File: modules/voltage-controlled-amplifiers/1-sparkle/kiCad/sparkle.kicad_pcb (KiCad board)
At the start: 2 copper layers, 90 x 111 mm, 83 parts, among them J1 OUT_1, J2 IN_1, J3 CV_1, J4 OUT_2, J5 IN_2, J6 CV_2, Q1 BC548, Q2 BC548, Q3 BC548, Q4 BC548, U1 TL074

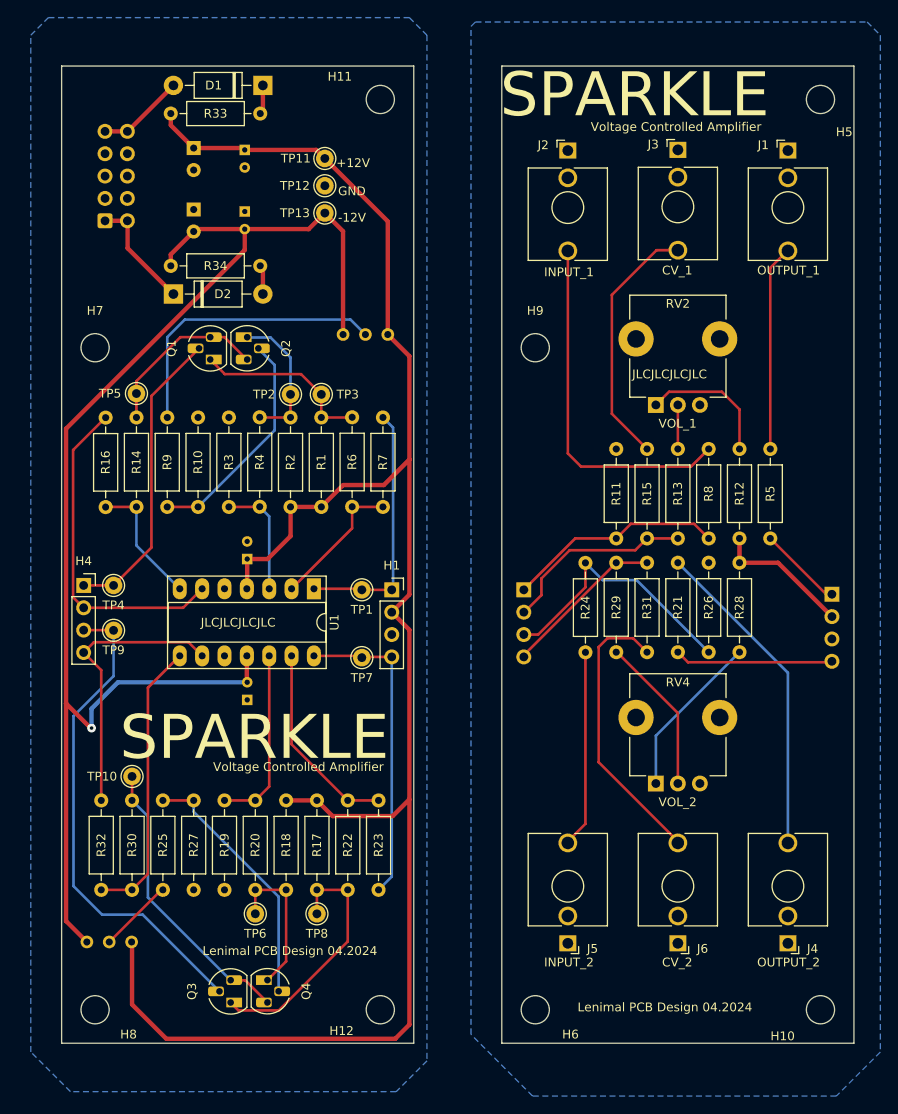
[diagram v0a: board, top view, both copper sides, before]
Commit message: add gerber files and ZIPs for V2
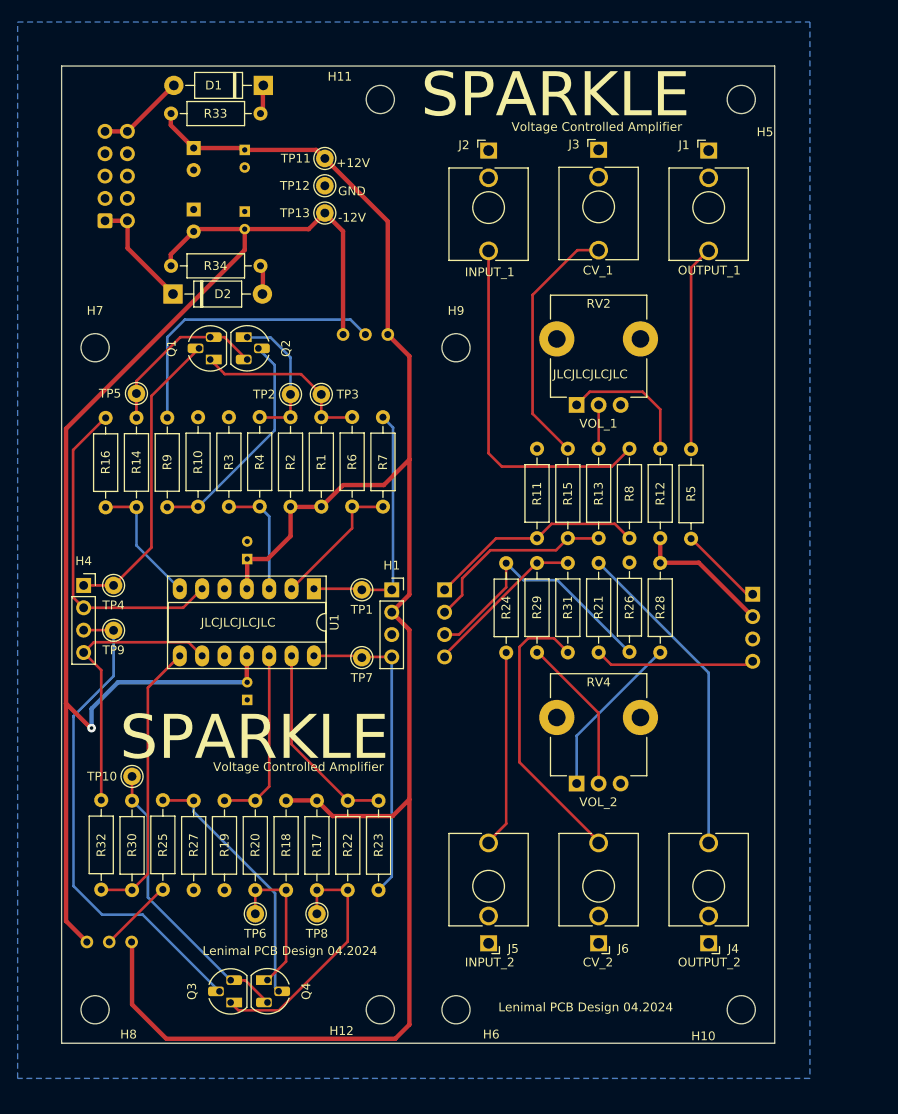
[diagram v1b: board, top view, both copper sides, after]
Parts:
- moved H2 9.00 mm to (128.5, 110.0)
- moved H3 9.00 mm to (93.5, 109.5)
- moved H6 9.00 mm to (94.8, 157.2)
- moved H9 9.00 mm to (94.8, 82.0)
- moved J1 9.00 mm to (123.5, 66.1)
- moved J2 9.00 mm to (98.5, 66.1)
- moved J3 9.00 mm to (111.0, 66.0)
- moved J4 9.00 mm to (123.5, 143.2)
- moved J5 9.00 mm to (98.5, 143.2)
- moved J6 9.00 mm to (111.0, 143.2)
- moved R11 9.00 mm to (104.0, 93.5)
- moved R12 9.00 mm to (118.0, 93.5)
- moved R13 9.00 mm to (111.0, 93.5)
- moved R15 9.00 mm to (107.5, 93.5)
- moved R21 9.00 mm to (111.0, 116.6)
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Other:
- board size 90 x 111 mm -> 81 x 111 mm
- board text added: "In the rack, a sparkle ignites, Voltage whispers, in the night. Amplifier, with power to soar, Sparkle's glow, forevermore."
- board text added: "Voltage flows, controlled and true, Sparkle's touch, a sonic hue. In every note, her brilliance gleams, Amplifying dreams, to realms unseen."
